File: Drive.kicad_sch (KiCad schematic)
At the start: 18 parts, among them Q1 CSD87333Q3D, U2 ACS711xEXLT-15AB

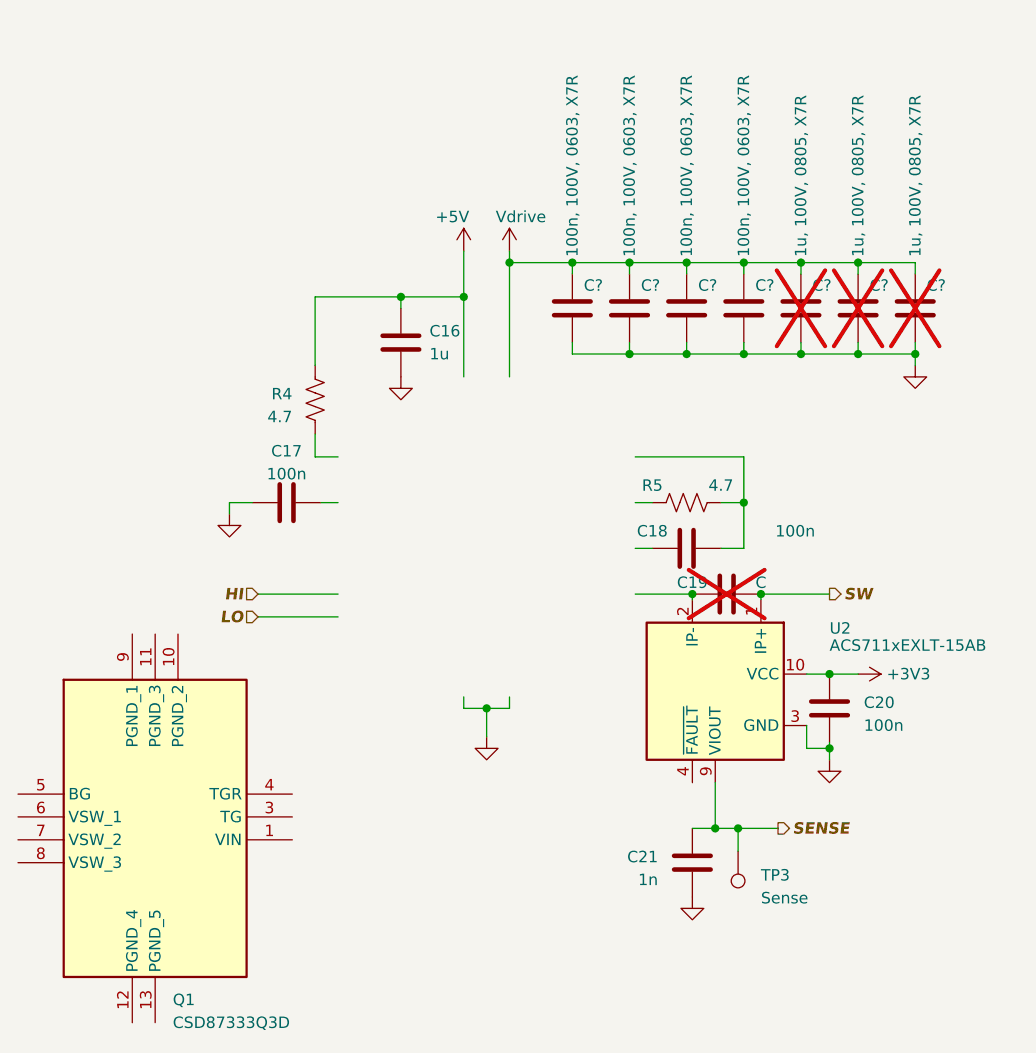
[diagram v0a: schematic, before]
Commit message: Update
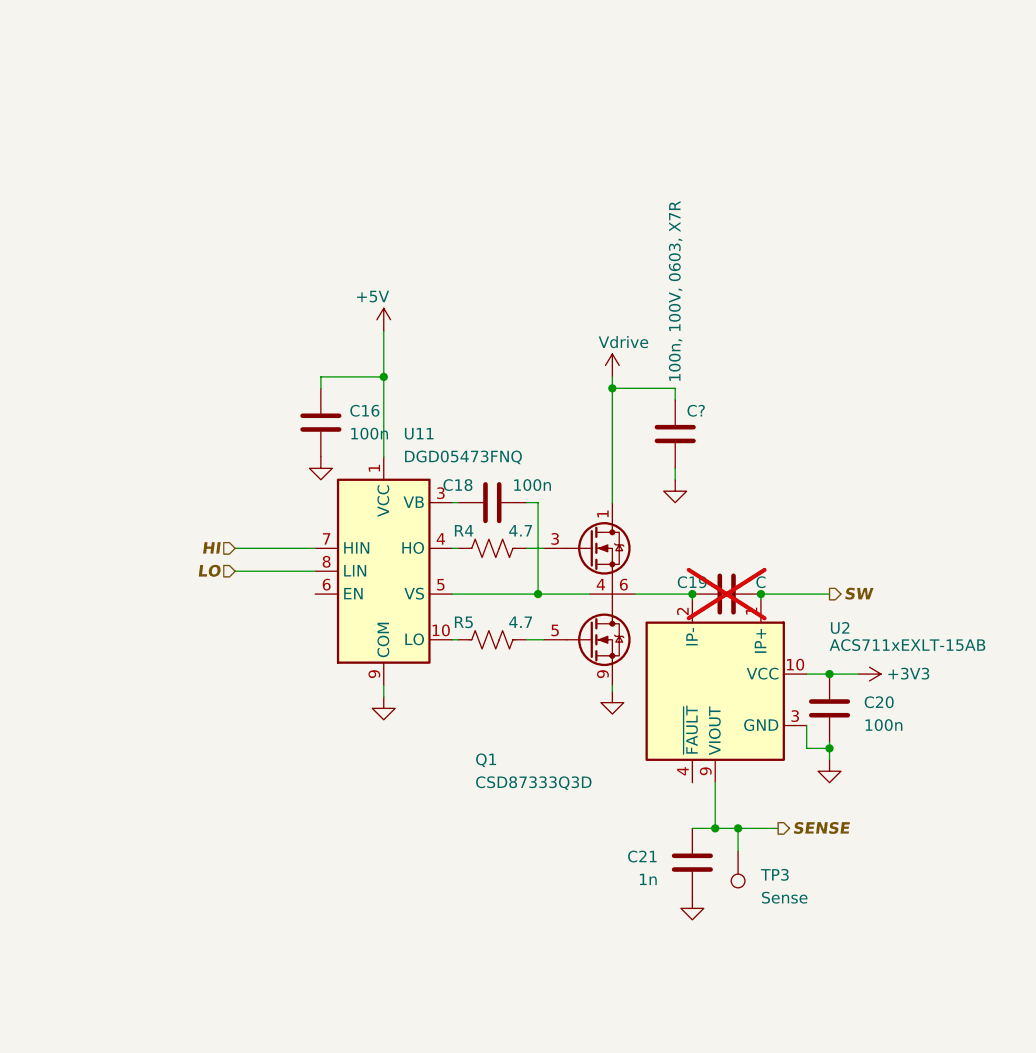
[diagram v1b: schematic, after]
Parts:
- removed C17: 100n, Capacitor_SMD:C_0402_1005Metric, symbol Device:C
- removed C? (x3): 100n, 100V, 0603, X7R, Capacitor_SMD:C_0603_1608Metric, symbol Device:C
- removed C? (x3): 1u, 100V, 0805, X7R, Capacitor_SMD:C_0805_2012Metric, symbol Device:C
- added U11: DGD05473FNQ, Package_DFN_QFN:DFN-10-1EP_3x3mm_P0.5mm_EP1.65x2.38mm, symbol Driver_FET:IR2106
- C16: value 1u -> 100n
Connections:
- net GND is gone; now on net EP: C16.2, C20.1, C21.1, C?.2, U2.3 (GND)
- net +5V: now also U11.1 (VCC); no longer R4.1
- net HI: now also U11.7 (HIN)
- net LO: now also U11.8 (LIN)
- net Vdrive: now also Q1.1 (VIN)
- net at R5.1: now also U11.10 (LO)
- net at R5.2: now also Q1.5 (BG); no longer C18.2
- net EP: now reaches Q1.10 (GND)
- net EP: now also Q1.11 (GND), Q1.12 (GND), Q1.13 (GND), Q1.9 (GND), U11.11 (EP), U11.9 (COM)
- net at Q1.3 (TG): now also R4.1
- net at Q1.4 (TGR): now also C18.2, U11.5 (VS)
- net at Q1.6 (SW): now also C19.1, Q1.7 (SW), Q1.8 (SW), U2.2 (IP-)
- net at C18.1: now also U11.3 (VB)
- net at R4.2: now also U11.4 (HO)
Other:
- moved on the sheet: C16, C18, C?, R4, R5
